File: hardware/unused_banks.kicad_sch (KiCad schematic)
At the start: 2 parts, among them U16 MPFS025T-FCVG484E, U9 MPFS025T-FCVG484E

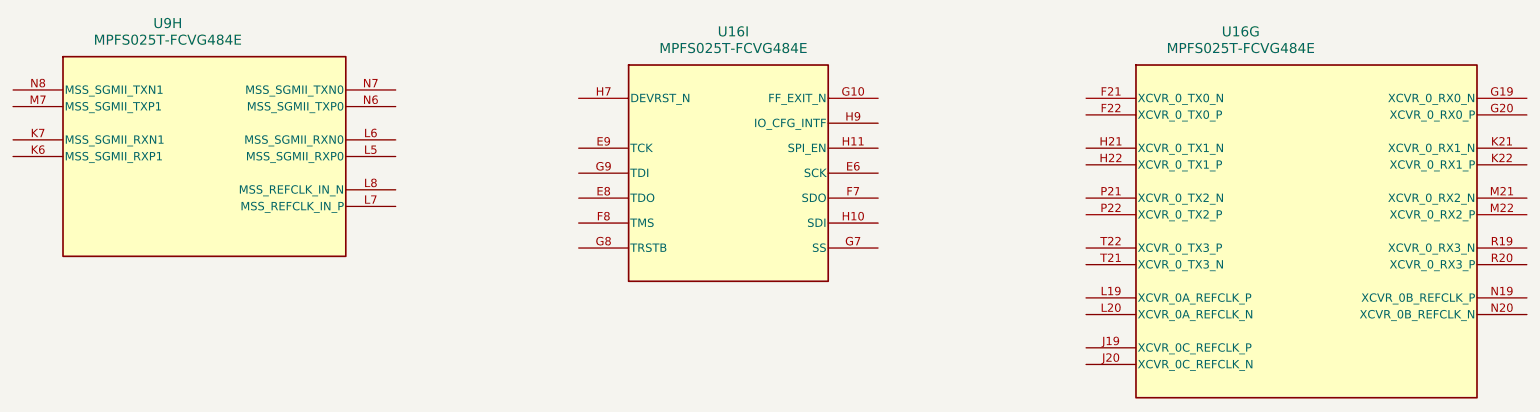
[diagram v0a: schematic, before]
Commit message: need finish io banks pinouts
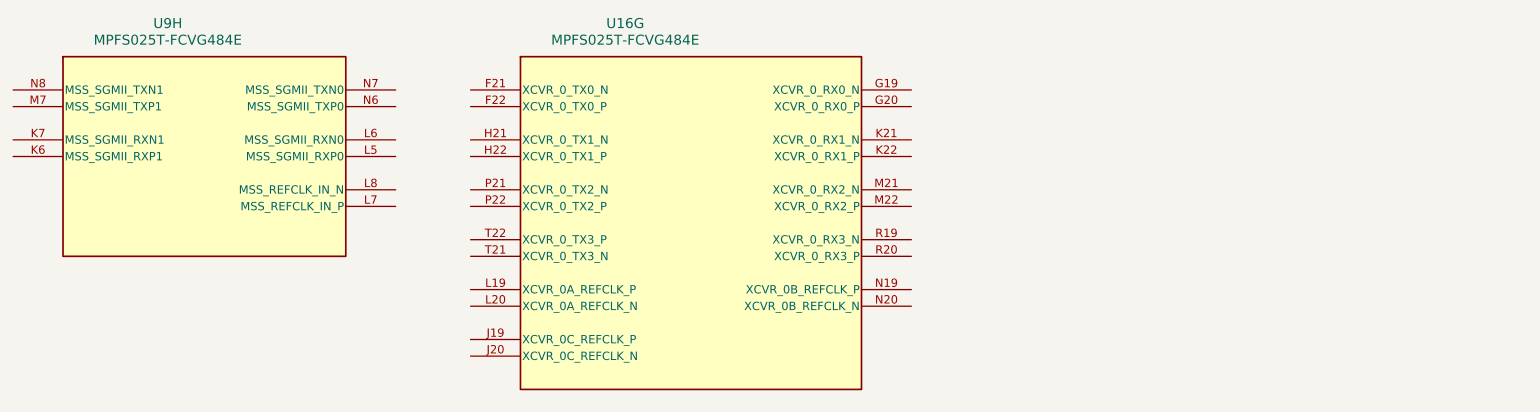
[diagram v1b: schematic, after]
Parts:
- removed unit 9 of U16
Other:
- moved on the sheet: U16G
